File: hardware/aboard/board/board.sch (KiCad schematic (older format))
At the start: 29 parts, among them J1 Conn_01x04_Male, P1 Power, P2 Analog, P3 Digital, P4 Digital, P5 CONN_01X01, P6 CONN_01X01, P7 CONN_01X01, P8 CONN_01X01, U1 24LC512, U10 ST25DV04K, U2 AT25SF081-SSHD-X, U3 24LC512, U4 AT25SF081-SSHD-X, U5 24LC512, U6 LTC3406ES5, U8 Si5351A, U9 ICE40UP5K-SG48ITR, Y1 Crystal

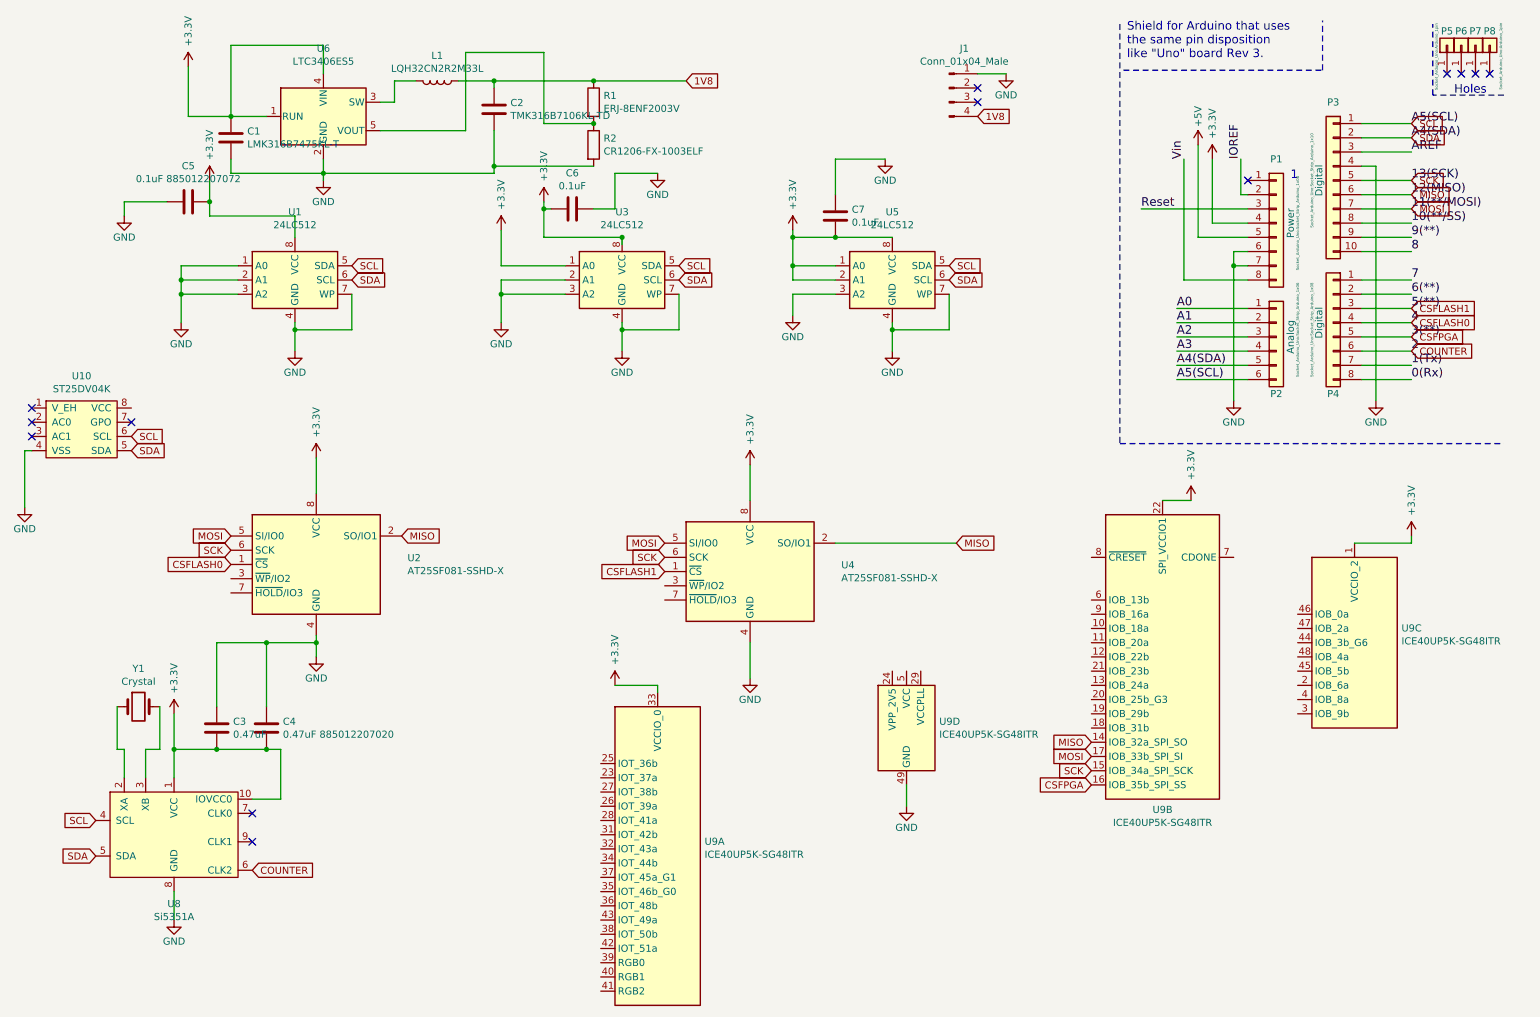
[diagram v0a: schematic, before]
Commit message: board for OM13088UL: process 3
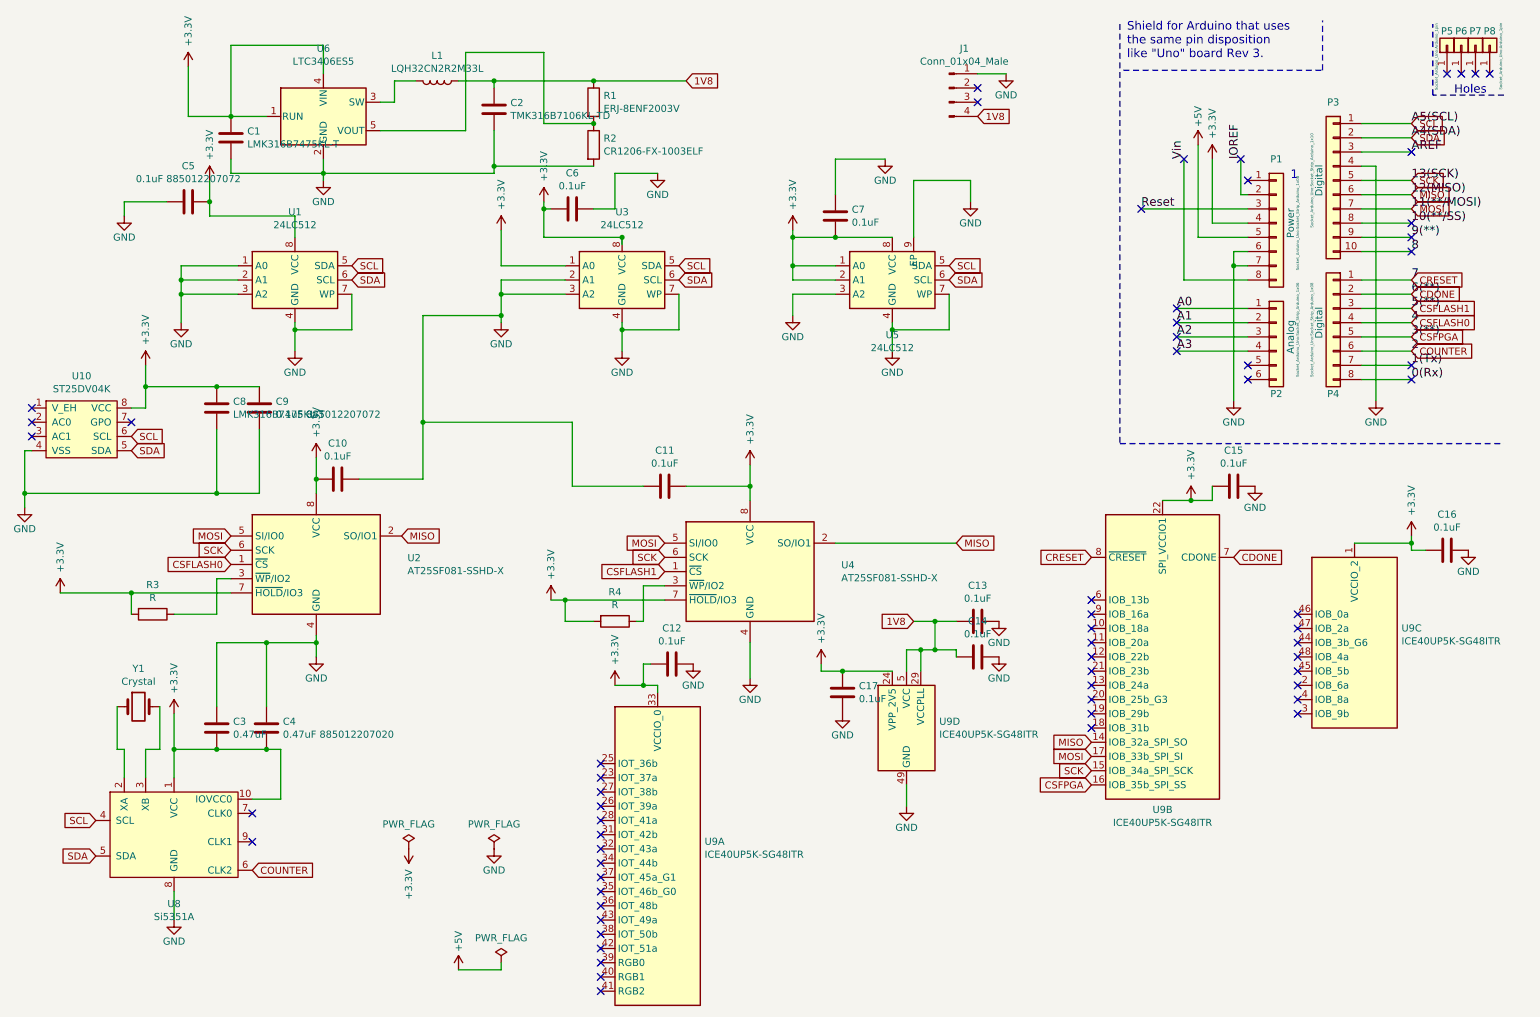
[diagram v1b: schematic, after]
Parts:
- removed U5: 24LC512, symbol Memory_EEPROM:24LC512
- added C10, C11, C12, C13, C14, C15, C16, C17: 0.1uF, Capacitor_SMD:C_0805_2012Metric, symbol Device:C
- added C8: LMK316B7475KL-T, Capacitor_SMD:C_1206_3216Metric, symbol Device:C
- added C9: 0.1uF 885012207072, Capacitor_SMD:C_0805_2012Metric, symbol Device:C
- added R3, R4: R, Resistor_SMD:R_1206_3216Metric, symbol Device:R
- added U5: 24LC512, Package_DFN_QFN:DFN-8-1EP_6x5mm_P1.27mm_EP4x4mm, symbol kilib2:24LC512
- U1, U10: footprint (none) -> Package_SO:TSSOP-8_4.4x3mm_P0.65mm
- U3: footprint (none) -> Package_SO:SOIC-8_3.9x4.9mm_P1.27mm
- U8: footprint (none) -> Package_SO:MSOP-10_3x3mm_P0.5mm
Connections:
- net 6(**) is gone; now on net CDONE: P4.2 (Pin_2)
- net 7 is gone; now on net CRESET: P4.1 (Pin_1)
- net +3V3: now also U10.8 (VCC), U2.7 (~HOLD~/IO3), U4.7 (~HOLD~/IO3), U9.24 (VPP_2V5), C10.2, C11.1, C12.2, C15.2, C16.2, C17.2, C8.1, C9.2, R3.2, R4.2, U5.1 (A0), U5.2 (A1), U5.8 (VCC)
- net 1V8: now also U9.29 (VCCPLL), U9.30 (VCC), U9.5 (VCC), C13.2, C14.2
- net GND: now also C10.1, C11.2, C12.1, C13.1, C14.1, C15.1, C16.1, C17.1, C8.2, C9.1, U5.3 (A2), U5.4 (GND), U5.7 (WP), U5.9 (EP)
- net SCL: now also U5.5 (SDA); no longer P2.6 (Pin_6)
- net SDA: now also U5.6 (SCL); no longer P2.5 (Pin_5)
- net at U2.3 (~WP~/IO2): now also R3.1
- net at U4.3 (~WP~/IO2): now also R4.1
- net CDONE: now reaches U9.7 (CDONE)
- net CRESET: now reaches U9.8 (~CRESET)
- no-connect marks 13 -> 63
